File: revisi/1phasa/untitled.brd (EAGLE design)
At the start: 80 x 102 mm, 52 parts, among them J1 U.FL-R-SMT(01), J2 10118193-0001LF, K1 SLA-05VDC-SL-C, Q1 S9013, Q16 MMBT3904, Q17 MMBT3904, Q18 12MHz, U1 AMS1117, U19 CH340G, U2 PC817X2NIP0F, U3 ESP32-WROOM-32D

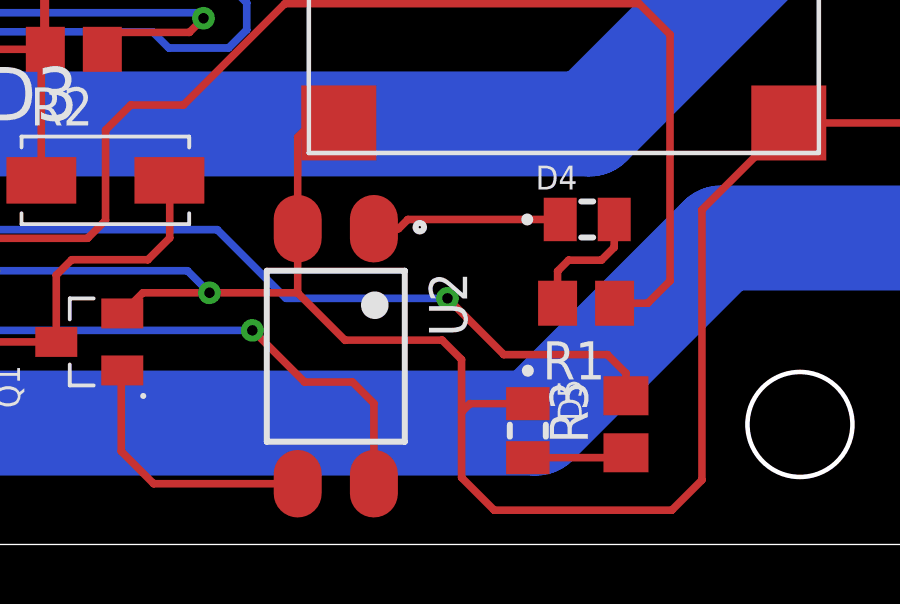
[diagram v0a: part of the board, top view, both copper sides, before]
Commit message: fix
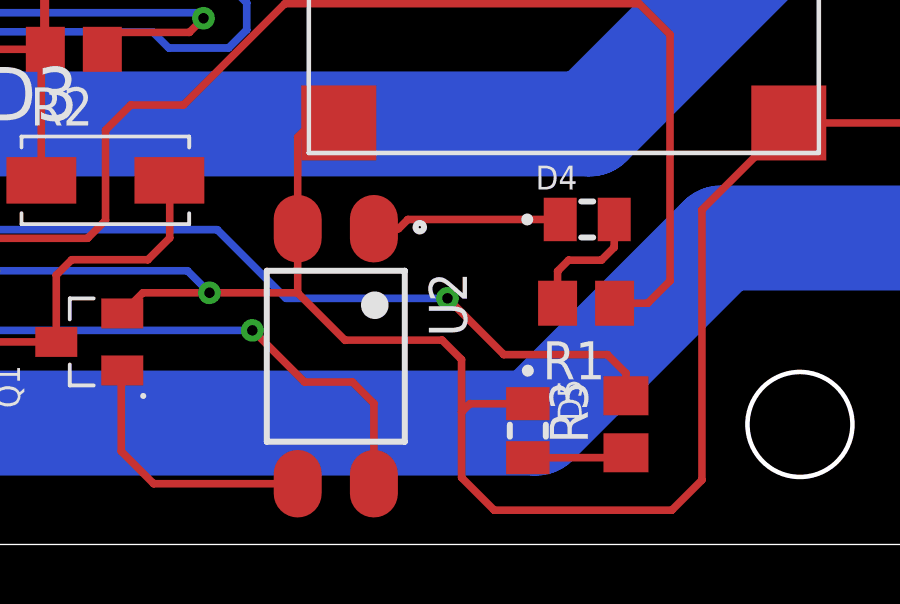
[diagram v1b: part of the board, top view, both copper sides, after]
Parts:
- R2, R3, R47: value 10k -> 1k
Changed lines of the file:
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@@
 <attribute name="VALUE" x="56.706540625" y="-0.418321875" size="1.27" layer="27" rot="R180"/>
 </element>
-<element name="R2" library="rcl" library_urn="urn:adsk.eagle:library:334" package="R0805" package3d_urn="urn:adsk.eagle:package:23553/2" value="10k" x="38.997128125" y="5.505603125" smashed="yes" rot="R180">
+<element name="R2" library="rcl" library_urn="urn:adsk.eagle:library:334" package="R0805" package3d_urn="urn:adsk.eagle:package:23553/2" value="1k" x="38.997128125" y="5.505603125" smashed="yes" rot="R180">
 <attribute name="NAME" x="39.632128125" y="4.235603125" size="1.27" layer="25" rot="R180"/>
 <attribute name="POPULARITY" value="86" x="-0.372871875" y="107.105603125" size="1.778" layer="27" rot="R180" display="off"/>
@@
 <attribute name="VALUE" x="28.455390625" y="76.59524375" size="1.27" layer="27" rot="R90"/>
 </element>
-<element name="R47" library="rcl" library_urn="urn:adsk.eagle:library:334" package="R0805" package3d_urn="urn:adsk.eagle:package:23553/2" value="10k" x="8.194" y="64.442871875" smashed="yes">
+<element name="R47" library="rcl" library_urn="urn:adsk.eagle:library:334" package="R0805" package3d_urn="urn:adsk.eagle:package:23553/2" value="1k" x="8.194" y="64.442871875" smashed="yes">
 <attribute name="NAME" x="7.559" y="65.712871875" size="1.27" layer="25"/>
 <attribute name="POPULARITY" value="86" x="37.404" y="-37.157128125" size="1.778" layer="27" display="off"/>
@@
 <attribute name="MF" value="Sharp Microelectronics" x="-36.09193125" y="-28.854778125" size="1.778" layer="27" rot="R270" display="off"/>
 <attribute name="MP" value="PC817X2NIP0F" x="-36.09193125" y="-28.854778125" size="1.778" layer="27" rot="R270" display="off"/>
+<attribute name="NAME" x="50.83386875" y="-1.9195375" size="1.27238125" layer="25" rot="R270"/>
 <attribute name="NAME" x="50.8300875" y="-1.922946875" size="1.27083125" layer="25" rot="R270"/>
-<attribute name="NAME" x="50.83386875" y="-1.9195375" size="1.27238125" layer="25" rot="R270"/>
 <attribute name="PACKAGE" value="SMD-4 Sharp Microelectronics" x="-36.09193125" y="-28.854778125" size="1.778" layer="27" rot="R270" display="off"/>
 <attribute name="PRICE" value="None" x="-36.09193125" y="-28.854778125" size="1.778" layer="27" rot="R270" display="off"/>
@@
 <attribute name="PURCHASE-URL" value="https://pricing.snapeda.com/search/part/SML-LXT0805IW-TR/?ref=eda" x="54.130403125" y="-7.20664375" size="1.778" layer="27" rot="R270" display="off"/>
 </element>
-<element name="R3" library="rcl" library_urn="urn:adsk.eagle:library:334" package="R0805" package3d_urn="urn:adsk.eagle:package:23553/2" value="10k" x="57.40076875" y="-6.994178125" smashed="yes" rot="R90">
+<element name="R3" library="rcl" library_urn="urn:adsk.eagle:library:334" package="R0805" package3d_urn="urn:adsk.eagle:package:23553/2" value="1k" x="57.40076875" y="-6.994178125" smashed="yes" rot="R90">
 <attribute name="NAME" x="56.13076875" y="-7.629178125" size="1.27" layer="25" rot="R90"/>
 <attribute name="POPULARITY" value="86" x="57.40076875" y="-6.994178125" size="1.778" layer="27" rot="R90" display="off"/>
